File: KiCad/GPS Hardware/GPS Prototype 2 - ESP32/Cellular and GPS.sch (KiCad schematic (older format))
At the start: 30 parts, among them J3 Conn_Coaxial, J6 SIM8065-6-1-14-01-A_REVA1, Q1 BC847, Q2 BC847, Q3 BSS84, U10 ublox_SAM-M8Q, U7 74AVC2T245GU-Q100X, U8 SARA-U201

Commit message: Update
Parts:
- D2: symbol GPS-Hardware-rescue:LED-Device -> GPS-Hardware-rescue:LED-Device-GPS-Hardware-rescue
- D3, D4, D5, D6: symbol GPS-Hardware-rescue:D_TVS-Device -> GPS-Hardware-rescue:D_TVS-Device-GPS-Hardware-rescue
- J3: symbol GPS-Hardware-rescue:Conn_Coaxial-Connector -> GPS-Hardware-rescue:Conn_Coaxial-Connector-GPS-Hardware-rescue
- Q1, Q2: symbol GPS-Hardware-rescue:BC847-Transistor_BJT -> GPS-Hardware-rescue:BC847-Transistor_BJT-GPS-Hardware-rescue
- Q3: symbol GPS-Hardware-rescue:BSS84-Transistor_FET -> GPS-Hardware-rescue:BSS84-Transistor_FET-GPS-Hardware-rescue
- U10: symbol GPS-Hardware-rescue:ublox_SAM-M8Q-RF_GPS -> GPS-Hardware-rescue:ublox_SAM-M8Q-RF_GPS-GPS-Hardware-rescue
- U8: symbol GPS-Hardware-rescue:SARA-U201-RF_GSM -> GPS-Hardware-rescue:SARA-U201-RF_GSM-GPS-Hardware-rescue
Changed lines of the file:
@@
 $EndDescr
 $Comp
-L GPS-Hardware-rescue:SARA-U201-RF_GSM U?
+L GPS-Hardware-rescue:SARA-U201-RF_GSM-GPS-Hardware-rescue U?
 U 1 1 6149258C
 P 3100 2850
@@
 CTS_Cellular
 $Comp
-L GPS-Hardware-rescue:GND-power #PWR?
+L GPS-Hardware-rescue:GND-power-GPS-Hardware-rescue #PWR?
 U 1 1 61492596
 P 2500 1950
@@
 $EndComp
 $Comp
-L GPS-Hardware-rescue:+1V8-power #PWR?
+L GPS-Hardware-rescue:+1V8-power-GPS-Hardware-rescue #PWR?
 U 1 1 6149259C
 P 3200 1750
@@
 	1600 2850 1700 2850
 $Comp
-L GPS-Hardware-rescue:+3V3-power #PWR?
+L GPS-Hardware-rescue:+3V3-power-GPS-Hardware-rescue #PWR?
 U 1 1 614925A6
 P 1700 2550
@@
 VCC
 $Comp
-L GPS-Hardware-rescue:GND-power #PWR?
+L GPS-Hardware-rescue:GND-power-GPS-Hardware-rescue #PWR?
 U 1 1 614925D1
 P 1850 1500
@@
 $EndComp
 $Comp
-L GPS-Hardware-rescue:GND-power #PWR?
+L GPS-Hardware-rescue:GND-power-GPS-Hardware-rescue #PWR?
 U 1 1 614925D7
 P 2150 1500
@@
 $EndComp
 $Comp
-L GPS-Hardware-rescue:GND-power #PWR?
+L GPS-Hardware-rescue:GND-power-GPS-Hardware-rescue #PWR?
 U 1 1 614925DD
 P 2450 1500
@@
 $EndComp
 $Comp
-L GPS-Hardware-rescue:GND-power #PWR?
+L GPS-Hardware-rescue:GND-power-GPS-Hardware-rescue #PWR?
 U 1 1 614925E3
 P 2750 1500
@@
 VCC
 $Comp
-L GPS-Hardware-rescue:Conn_Coaxial-Connector J?
+L GPS-Hardware-rescue:Conn_Coaxial-Connector-GPS-Hardware-rescue J?
 U 1 1 614925ED
 P 3900 1950
@@
 $EndComp
 $Comp
-L GPS-Hardware-rescue:ublox_SAM-M8Q-RF_GPS U10
+L GPS-Hardware-rescue:ublox_SAM-M8Q-RF_GPS-GPS-Hardware-rescue U10
 U 1 1 614F3B93
 P 6000 6250
@@
 $EndComp
 $Comp
-L GPS-Hardware-rescue:GND-power #PWR0171
+L GPS-Hardware-rescue:GND-power-GPS-Hardware-rescue #PWR0171
 U 1 1 6152BD4B
 P 2300 5800
@@
 $EndComp
 $Comp
-L GPS-Hardware-rescue:GND-power #PWR0172
+L GPS-Hardware-rescue:GND-power-GPS-Hardware-rescue #PWR0172
 U 1 1 6152F81D
 P 2300 5600
@@
 $EndComp
 $Comp
-L GPS-Hardware-rescue:GND-power #PWR0173
+L GPS-Hardware-rescue:GND-power-GPS-Hardware-rescue #PWR0173
 U 1 1 6153C648
 P 3300 6000
@@
 	3200 5700 3300 5700
 $Comp
-L GPS-Hardware-rescue:+1V8-power #PWR0174
+L GPS-Hardware-rescue:+1V8-power-GPS-Hardware-rescue #PWR0174
 U 1 1 6153DDB4
 P 3400 5700
@@
 	3200 5600 3950 5600
 $Comp
-L GPS-Hardware-rescue:GND-power #PWR0175
+L GPS-Hardware-rescue:GND-power-GPS-Hardware-rescue #PWR0175
 U 1 1 61540A2C
 P 3950 5900
@@
 Connection ~ 3950 5600
 $Comp
-L GPS-Hardware-rescue:GND-power #PWR0176
+L GPS-Hardware-rescue:GND-power-GPS-Hardware-rescue #PWR0176
 U 1 1 61553C2B
 P 3200 6250
@@
 TX_GPS
 $Comp
-L GPS-Hardware-rescue:GND-power #PWR0177
+L GPS-Hardware-rescue:GND-power-GPS-Hardware-rescue #PWR0177
 U 1 1 61577124
 P 6000 6750
@@
 $EndComp
 $Comp
-L GPS-Hardware-rescue:GND-power #PWR0178
+L GPS-Hardware-rescue:GND-power-GPS-Hardware-rescue #PWR0178
 U 1 1 61579240
 P 5600 5700
@@
 NoConn ~ 2500 3750
 $Comp
-L GPS-Hardware-rescue:GND-power #PWR0179
+L GPS-Hardware-rescue:GND-power-GPS-Hardware-rescue #PWR0179
 U 1 1 615C3FBF
 P 3100 3950
@@
 $EndComp
 $Comp
-L GPS-Hardware-rescue:BC847-Transistor_BJT Q1
+L GPS-Hardware-rescue:BC847-Transistor_BJT-GPS-Hardware-rescue Q1
 U 1 1 615DCAB0
 P 4350 2850
@@
 $EndComp
 $Comp
-L GPS-Hardware-rescue:LED-Device D2
+L GPS-Hardware-rescue:LED-Device-GPS-Hardware-rescue D2
 U 1 1 615DFC25
 P 4450 2500
@@
 	3750 2850 3700 2850
 $Comp
-L GPS-Hardware-rescue:GND-power #PWR0180
+L GPS-Hardware-rescue:GND-power-GPS-Hardware-rescue #PWR0180
 U 1 1 615E6884
 P 4450 3050
@@
 $EndComp
 $Comp
-L GPS-Hardware-rescue:GND-power #PWR0181
+L GPS-Hardware-rescue:GND-power-GPS-Hardware-rescue #PWR0181
 U 1 1 615E6F5B
 P 4100 3150
@@
 VSIM
 $Comp
-L GPS-Hardware-rescue:GND-power #PWR0113
+L GPS-Hardware-rescue:GND-power-GPS-Hardware-rescue #PWR0113
 U 1 1 61244203
 P 3900 1750
@@
 $EndComp
 $Comp
-L GPS-Hardware-rescue:GND-power #PWR0114
+L GPS-Hardware-rescue:GND-power-GPS-Hardware-rescue #PWR0114
 U 1 1 61320761
 P 7850 4250
@@
 $EndComp
 $Comp
-L GPS-Hardware-rescue:GND-power #PWR0128
+L GPS-Hardware-rescue:GND-power-GPS-Hardware-rescue #PWR0128
 U 1 1 61320767
 P 8350 4450
@@
 $EndComp
 $Comp
-L GPS-Hardware-rescue:GND-power #PWR0129
+L GPS-Hardware-rescue:GND-power-GPS-Hardware-rescue #PWR0129
 U 1 1 6132076D
 P 8250 5300
@@
 $EndComp
 $Comp
-L GPS-Hardware-rescue:GND-power #PWR0133
+L GPS-Hardware-rescue:GND-power-GPS-Hardware-rescue #PWR0133
 U 1 1 61320773
 P 7550 4350
@@
 $EndComp
 $Comp
-L GPS-Hardware-rescue:GND-power #PWR0157
+L GPS-Hardware-rescue:GND-power-GPS-Hardware-rescue #PWR0157
 U 1 1 61320779
 P 8200 4250
@@
 $EndComp
 $Comp
-L GPS-Hardware-rescue:GND-power #PWR0158
+L GPS-Hardware-rescue:GND-power-GPS-Hardware-rescue #PWR0158
 U 1 1 6132077F
 P 7950 5500
@@
 RST
 $Comp
-L GPS-Hardware-rescue:D_TVS-Device D3
+L GPS-Hardware-rescue:D_TVS-Device-GPS-Hardware-rescue D3
 U 1 1 61320797
 P 7850 4100
@@
 $EndComp
 $Comp
-L GPS-Hardware-rescue:D_TVS-Device D5
+L GPS-Hardware-rescue:D_TVS-Device-GPS-Hardware-rescue D5
 U 1 1 6132079D
 P 8250 5150
@@
 $EndComp
 $Comp
-L GPS-Hardware-rescue:D_TVS-Device D4
+L GPS-Hardware-rescue:D_TVS-Device-GPS-Hardware-rescue D4
 U 1 1 613207AF
 P 8350 4600
@@
 VSIM
 $Comp
-L GPS-Hardware-rescue:GND-power #PWR0159
+L GPS-Hardware-rescue:GND-power-GPS-Hardware-rescue #PWR0159
 U 1 1 61330E52
 P 8000 3550
@@
 $EndComp
 $Comp
-L GPS-Hardware-rescue:GND-power #PWR0160
+L GPS-Hardware-rescue:GND-power-GPS-Hardware-rescue #PWR0160
 U 1 1 61330E58
 P 7700 3550
@@
 $EndComp
 $Comp
-L GPS-Hardware-rescue:GND-power #PWR0161
+L GPS-Hardware-rescue:GND-power-GPS-Hardware-rescue #PWR0161
 U 1 1 61330E5E
 P 7350 3550
@@
 Connection ~ 8000 3850
 $Comp
-L GPS-Hardware-rescue:D_TVS-Device D6
+L GPS-Hardware-rescue:D_TVS-Device-GPS-Hardware-rescue D6
 U 1 1 61330E66
 P 8000 3700
@@
 $EndComp
 $Comp
-L GPS-Hardware-rescue:GND-power #PWR0162
+L GPS-Hardware-rescue:GND-power-GPS-Hardware-rescue #PWR0162
 U 1 1 61331880
 P 8650 4150
@@
 $EndComp
 $Comp
-L GPS-Hardware-rescue:BC847-Transistor_BJT Q2
+L GPS-Hardware-rescue:BC847-Transistor_BJT-GPS-Hardware-rescue Q2
 U 1 1 613C6B7F
 P 5050 4050
@@
 	4750 4050 4850 4050
 $Comp
-L GPS-Hardware-rescue:GND-power #PWR0104
+L GPS-Hardware-rescue:GND-power-GPS-Hardware-rescue #PWR0104
 U 1 1 613D3752
 P 5150 4350
@@
 	5150 3750 5150 3800
 $Comp
-L GPS-Hardware-rescue:+3V3-power #PWR0163
+L GPS-Hardware-rescue:+3V3-power-GPS-Hardware-rescue #PWR0163
 U 1 1 613DE378
 P 5150 3350
@@
 	5150 3450 5150 3350
 $Comp
-L GPS-Hardware-rescue:BSS84-Transistor_FET Q3
+L GPS-Hardware-rescue:BSS84-Transistor_FET-GPS-Hardware-rescue Q3
 U 1 1 613E1FB9
 P 5650 3800

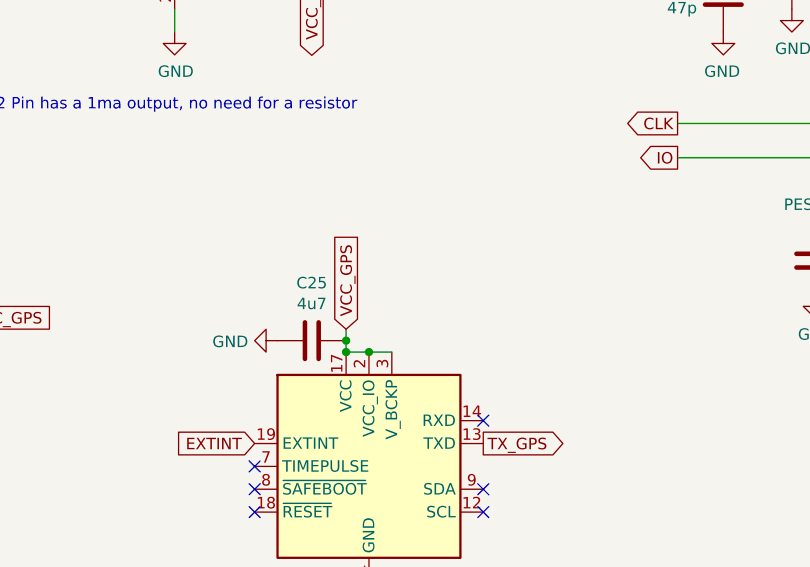
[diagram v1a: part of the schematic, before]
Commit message: Update to Laptop
Still a lot more to go
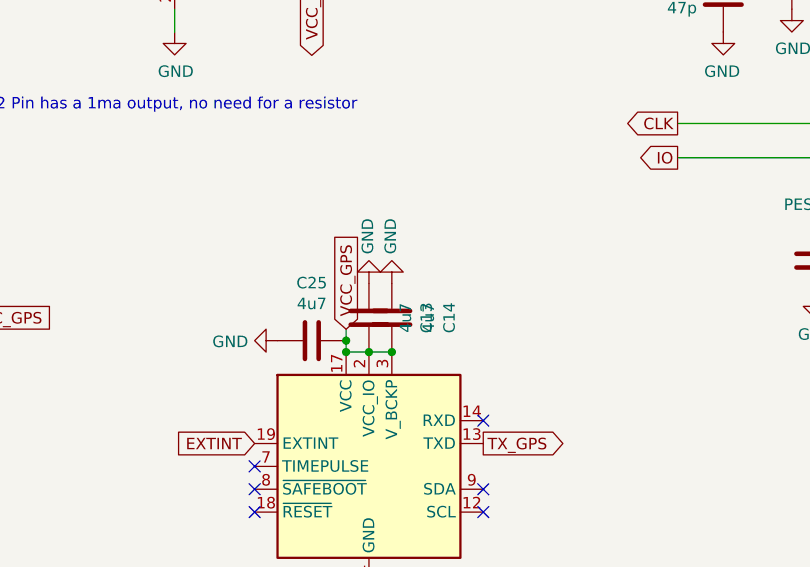
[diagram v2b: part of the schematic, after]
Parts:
- added C13, C14: 4u7, Capacitor_SMD:C_1206_3216Metric_Pad1.33x1.80mm_HandSolder, symbol GPS-Hardware-rescue:C-Device
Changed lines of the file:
@@
 NoConn ~ 8650 4450
 NoConn ~ 8650 4250
+$Comp
+L GPS-Hardware-rescue:C-Device C13
+U 1 1 62C636CA
+P 6000 5600
+F 0 "C13" V 5748 5600 50  0000 C CNN
+F 1 "4u7" V 5839 5600 50  0000 C CNN
+F 2 "Capacitor_SMD:C_1206_3216Metric_Pad1.33x1.80mm_HandSolder" H 6038 5450 50  0001 C CNN
+F 3 "~" H 6000 5600 50  0001 C CNN
+	1    6000 5600
+	-1   0    0    1
+$EndComp
+$Comp
+L GPS-Hardware-rescue:C-Device C14
+U 1 1 62C6483D
+P 6100 5600
+F 0 "C14" V 5848 5600 50  0000 C CNN
+F 1 "4u7" V 5939 5600 50  0000 C CNN
+F 2 "Capacitor_SMD:C_1206_3216Metric_Pad1.33x1.80mm_HandSolder" H 6138 5450 50  0001 C CNN
+F 3 "~" H 6100 5600 50  0001 C CNN
+	1    6100 5600
+	-1   0    0    1
+$EndComp
+Connection ~ 6100 5750
+$Comp
+L GPS-Hardware-rescue:GND-power-GPS-Hardware-rescue #PWR07
+U 1 1 62C65505
+P 6000 5450
+F 0 "#PWR07" H 6000 5200 50  0001 C CNN
+F 1 "GND" V 6005 5322 50  0000 R CNN
+F 2 "" H 6000 5450 50  0001 C CNN
+F 3 "" H 6000 5450 50  0001 C CNN
+	1    6000 5450
+	-1   0    0    1
+$EndComp
+$Comp
+L GPS-Hardware-rescue:GND-power-GPS-Hardware-rescue #PWR08
+U 1 1 62C65DF6
+P 6100 5450
+F 0 "#PWR08" H 6100 5200 50  0001 C CNN
+F 1 "GND" V 6105 5322 50  0000 R CNN
+F 2 "" H 6100 5450 50  0001 C CNN
+F 3 "" H 6100 5450 50  0001 C CNN
+	1    6100 5450
+	-1   0    0    1
+$EndComp
 $EndSCHEMATC

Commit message: Update to laptop
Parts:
- removed D3, D4, D5, D6: PESD0402, Capacitor_SMD:C_0402_1005Metric_Pad0.74x0.62mm_HandSolder, symbol GPS-Hardware-rescue:D_TVS-Device-GPS-Hardware-rescue
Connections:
- wire segments 50 -> 45
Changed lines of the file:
@@
-$EndComp
-$Comp
-L GPS-Hardware-rescue:GND-power-GPS-Hardware-rescue #PWR0114
-U 1 1 61320761
-P 7850 4250
-F 0 "#PWR0114" H 7850 4000 50  0001 C CNN
-F 1 "GND" H 7855 4077 50  0000 C CNN
-F 2 "" H 7850 4250 50  0001 C CNN
-F 3 "" H 7850 4250 50  0001 C CNN
-	1    7850 4250
-	1    0    0    -1
-$EndComp
-$Comp
-L GPS-Hardware-rescue:GND-power-GPS-Hardware-rescue #PWR0128
-U 1 1 61320767
-P 8350 4450
-F 0 "#PWR0128" H 8350 4200 50  0001 C CNN
-F 1 "GND" H 8355 4277 50  0000 C CNN
-F 2 "" H 8350 4450 50  0001 C CNN
-F 3 "" H 8350 4450 50  0001 C CNN
-	1    8350 4450
-	-1   0    0    1
-$EndComp
-$Comp
-L GPS-Hardware-rescue:GND-power-GPS-Hardware-rescue #PWR0129
-U 1 1 6132076D
-P 8250 5300
-F 0 "#PWR0129" H 8250 5050 50  0001 C CNN
-F 1 "GND" H 8255 5127 50  0000 C CNN
-F 2 "" H 8250 5300 50  0001 C CNN
-F 3 "" H 8250 5300 50  0001 C CNN
-	1    8250 5300
-	1    0    0    -1
 $EndComp
 $Comp
@@
 Connection ~ 7550 3950
 Wire Wire Line
-	8250 5000 8250 4900
-Wire Wire Line
-	8250 4900 7950 4900
-Connection ~ 8250 4900
-Wire Wire Line
 	7950 5200 7950 4900
 Text GLabel 7350 4750 0    50   Output ~ 0
@@
 Text GLabel 7350 3950 0    50   Output ~ 0
 RST
-$Comp
-L GPS-Hardware-rescue:D_TVS-Device-GPS-Hardware-rescue D3
-U 1 1 61320797
-P 7850 4100
-F 0 "D3" V 7804 4180 50  0000 L CNN
-F 1 "PESD0402" V 7895 4180 50  0000 L CNN
-F 2 "Capacitor_SMD:C_0402_1005Metric_Pad0.74x0.62mm_HandSolder" H 7850 4100 50  0001 C CNN
-F 3 "~" H 7850 4100 50  0001 C CNN
-	1    7850 4100
-	0    -1   -1   0
-$EndComp
-$Comp
-L GPS-Hardware-rescue:D_TVS-Device-GPS-Hardware-rescue D5
-U 1 1 6132079D
-P 8250 5150
-F 0 "D5" V 8204 5230 50  0000 L CNN
-F 1 "PESD0402" V 8295 5230 50  0000 L CNN
-F 2 "Capacitor_SMD:C_0402_1005Metric_Pad0.74x0.62mm_HandSolder" H 8250 5150 50  0001 C CNN
-F 3 "~" H 8250 5150 50  0001 C CNN
-	1    8250 5150
-	0    -1   -1   0
-$EndComp
 $Comp
 L GPS-Hardware-rescue:C-Device C28
@@
 	1    7950 5350
 	1    0    0    -1
-$EndComp
-$Comp
-L GPS-Hardware-rescue:D_TVS-Device-GPS-Hardware-rescue D4
-U 1 1 613207AF
-P 8350 4600
-F 0 "D4" V 8304 4680 50  0000 L CNN
-F 1 "PESD0402" V 8395 4680 50  0000 L CNN
-F 2 "Capacitor_SMD:C_0402_1005Metric_Pad0.74x0.62mm_HandSolder" H 8350 4600 50  0001 C CNN
-F 3 "~" H 8350 4600 50  0001 C CNN
-	1    8350 4600
-	0    1    1    0
 $EndComp
 $Comp
@@
 VSIM
 $Comp
-L GPS-Hardware-rescue:GND-power-GPS-Hardware-rescue #PWR0159
-U 1 1 61330E52
-P 8000 3550
-F 0 "#PWR0159" H 8000 3300 50  0001 C CNN
-F 1 "GND" H 8005 3377 50  0000 C CNN
-F 2 "" H 8000 3550 50  0001 C CNN
-F 3 "" H 8000 3550 50  0001 C CNN
-	1    8000 3550
-	1    0    0    1
-$EndComp
-$Comp
 L GPS-Hardware-rescue:GND-power-GPS-Hardware-rescue #PWR0160
 U 1 1 61330E58
@@
 	1    0    0    1
 $EndComp
-Connection ~ 8000 3850
-$Comp
-L GPS-Hardware-rescue:D_TVS-Device-GPS-Hardware-rescue D6
-U 1 1 61330E66
-P 8000 3700
-F 0 "D6" V 7954 3780 50  0000 L CNN
-F 1 "PESD0402" V 8045 3780 50  0000 L CNN
-F 2 "Capacitor_SMD:C_0402_1005Metric_Pad0.74x0.62mm_HandSolder" H 8000 3700 50  0001 C CNN
-F 3 "~" H 8000 3700 50  0001 C CNN
-	1    8000 3700
-	0    1    -1   0
-$EndComp
 $Comp
 L GPS-Hardware-rescue:C-Device C31
@@
 	1    0    0    1
 $EndComp
-Wire Wire Line
-	7700 3850 8000 3850
 Wire Wire Line
 	7350 3850 7700 3850
@@
 $EndComp
 Wire Wire Line
-	8000 3850 8650 3850
-Connection ~ 7850 3950
-Wire Wire Line
-	7850 3950 7550 3950
-Wire Wire Line
-	7850 3950 8650 3950
-Wire Wire Line
 	7350 4750 8200 4750
 Wire Wire Line
@@
 Connection ~ 8200 4750
 Wire Wire Line
-	8200 4750 8350 4750
-Wire Wire Line
-	8350 4750 8500 4750
-Wire Wire Line
 	8500 4750 8500 4050
 Wire Wire Line
 	8500 4050 8650 4050
-Connection ~ 8350 4750
 Connection ~ 7950 4900
 Wire Wire Line
@@
 Wire Wire Line
 	8600 4350 8650 4350
-Wire Wire Line
-	8250 4900 8600 4900
 NoConn ~ 8650 4450
 NoConn ~ 8650 4250
@@
 	-1   0    0    1
 $EndComp
+Wire Wire Line
+	7700 3850 8650 3850
+Wire Wire Line
+	7550 3950 8650 3950
+Wire Wire Line
+	8200 4750 8500 4750
+Wire Wire Line
+	7950 4900 8600 4900
 $EndSCHEMATC

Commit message: Update
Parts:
- removed Q2: BC847, Package_TO_SOT_SMD:SOT-23, symbol GPS-Hardware-rescue:BC847-Transistor_BJT-GPS-Hardware-rescue
- removed Q3: BSS84, Package_TO_SOT_SMD:SOT-323_SC-70, symbol GPS-Hardware-rescue:BSS84-Transistor_FET-GPS-Hardware-rescue
- removed R20: 47k, Resistor_SMD:R_1206_3216Metric_Pad1.30x1.75mm_HandSolder, symbol GPS-Hardware-rescue:R-Device
- added D3: LED, LED_SMD:LED_1206_3216Metric_Pad1.42x1.75mm_HandSolder, symbol Device:LED
- added Q2: 2N7002, Package_TO_SOT_SMD:SOT-23, symbol Transistor_FET:2N7002
- added R15: 1k, Resistor_SMD:R_1206_3216Metric_Pad1.30x1.75mm_HandSolder, symbol Device:R
- R19: value 250 -> 820
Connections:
- net labels removed: GPIO2, VCC_GPS
- wire segments 45 -> 39
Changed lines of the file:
@@
 	1    0    0    -1
 $EndComp
-Text GLabel 2500 3050 0    50   Output ~ 0
+Text GLabel 1400 3250 0    50   Output ~ 0
 RESET_Cellular
 Wire Wire Line
@@
 	1    0    0    -1
 $EndComp
-Text GLabel 3700 2950 2    50   Output ~ 0
-GPIO2
 $Comp
 L GPS~Hardware:74AVC2T245GU-Q100X U7
@@
 	0    1    1    0
 $EndComp
-Text GLabel 1900 5500 1    50   Input ~ 0
-VCC_GPS
 Wire Wire Line
 	1900 5500 1900 5700
@@
 	1    0    0    -1
 $EndComp
-Text GLabel 4200 5600 2    50   Input ~ 0
-VCC_GPS
 Wire Wire Line
 	4200 5600 3950 5600
@@
 Wire Wire Line
 	5900 5700 5900 5750
-Text GLabel 5900 5650 1    50   Input ~ 0
-VCC_GPS
 Wire Wire Line
 	6100 5750 6000 5750
@@
 Connection ~ 6000 5750
 Connection ~ 5900 5750
-NoConn ~ 5500 6250
 NoConn ~ 5500 6350
 NoConn ~ 5500 6450
@@
 AR Path="/613BCFF5/615E2B7B" Ref="R19"  Part="1"
 F 0 "R19" H 4520 2246 50  0000 L CNN
-F 1 "250" V 4450 2150 50  0000 L CNN
+F 1 "820" V 4450 2150 50  0000 L CNN
 F 2 "Resistor_SMD:R_1206_3216Metric_Pad1.30x1.75mm_HandSolder" V 4380 2200 50  0001 C CNN
 F 3 "~" H 4450 2200 50  0001 C CNN
@@
 	0    1    1    0
 $EndComp
-$Comp
-L GPS-Hardware-rescue:BC847-Transistor_BJT-GPS-Hardware-rescue Q2
-U 1 1 613C6B7F
-P 5050 4050
-F 0 "Q2" H 5241 4096 50  0000 L CNN
-F 1 "BC847" H 5241 4005 50  0000 L CNN
-F 2 "Package_TO_SOT_SMD:SOT-23" H 5250 3975 50  0001 L CIN
-F 3 "https://www.mouser.co.uk/datasheet/2/308/1/BC846ALT1_D-2310268.pdf" H 5050 4050 50  0001 L CNN
-	1    5050 4050
-	1    0    0    -1
-$EndComp
-Text GLabel 4750 4050 0    50   Input ~ 0
-GPIO2
-Wire Wire Line
-	4750 4050 4850 4050
-$Comp
-L GPS-Hardware-rescue:GND-power-GPS-Hardware-rescue #PWR0104
-U 1 1 613D3752
-P 5150 4350
-F 0 "#PWR0104" H 5150 4100 50  0001 C CNN
-F 1 "GND" H 5155 4177 50  0000 C CNN
-F 2 "" H 5150 4350 50  0001 C CNN
-F 3 "" H 5150 4350 50  0001 C CNN
-	1    5150 4350
-	1    0    0    -1
-$EndComp
-Wire Wire Line
-	5150 4250 5150 4350
-$Comp
-L GPS-Hardware-rescue:R-Device R20
-U 1 1 613D777A
-P 5150 3600
-F 0 "R20" H 5220 3646 50  0000 L CNN
-F 1 "47k" H 5220 3555 50  0000 L CNN
-F 2 "Resistor_SMD:R_1206_3216Metric_Pad1.30x1.75mm_HandSolder" V 5080 3600 50  0001 C CNN
-F 3 "~" H 5150 3600 50  0001 C CNN
-	1    5150 3600
-	1    0    0    -1
-$EndComp
-Wire Wire Line
-	5150 3750 5150 3800
-$Comp
-L GPS-Hardware-rescue:+3V3-power-GPS-Hardware-rescue #PWR0163
-U 1 1 613DE378
-P 5150 3350
-F 0 "#PWR0163" H 5150 3200 50  0001 C CNN
-F 1 "+3V3" H 5165 3523 50  0000 C CNN
-F 2 "" H 5150 3350 50  0001 C CNN
-F 3 "" H 5150 3350 50  0001 C CNN
-	1    5150 3350
-	1    0    0    -1
-$EndComp
-Wire Wire Line
-	5150 3450 5150 3350
-$Comp
-L GPS-Hardware-rescue:BSS84-Transistor_FET-GPS-Hardware-rescue Q3
-U 1 1 613E1FB9
-P 5650 3800
-F 0 "Q3" H 5854 3754 50  0000 L CNN
-F 1 "BSS84" H 5854 3845 50  0000 L CNN
-F 2 "Package_TO_SOT_SMD:SOT-323_SC-70" H 5850 3725 50  0001 L CIN
-F 3 "http://assets.nexperia.com/documents/data-sheet/BSS84.pdf" H 5650 3800 50  0001 L CNN
-	1    5650 3800
-	1    0    0    1
-$EndComp
-Wire Wire Line
-	5450 3800 5150 3800
-Connection ~ 5150 3800
-Wire Wire Line
-	5150 3800 5150 3850
-Wire Wire Line
-	5150 3450 5750 3450
-Wire Wire Line
-	5750 3450 5750 3600
-Connection ~ 5150 3450
-Text GLabel 5750 4050 3    50   Output ~ 0
-VCC_GPS
-Wire Wire Line
-	5750 4000 5750 4050
-Text Notes 4200 4700 0    50   ~ 0
+Text Notes 5050 2850 0    50   ~ 0
 GPIO2 Pin has a 1ma output, no need for a resistor
 $Comp
@@
 Wire Wire Line
 	7950 4900 8600 4900
+NoConn ~ 3700 2950
+$Comp
+L GPS-Hardware-rescue:+3V3-power-GPS-Hardware-rescue #PWR?
+U 1 1 62EFB8D4
+P 1900 5500
+AR Path="/613BCFBA/62EFB8D4" Ref="#PWR?"  Part="1"
+AR Path="/613BCFF5/62EFB8D4" Ref="#PWR0114"  Part="1"
+F 0 "#PWR0114" H 1900 5350 50  0001 C CNN
+F 1 "+3V3" H 1915 5673 50  0000 C CNN
+F 2 "" H 1900 5500 50  0001 C CNN
+F 3 "" H 1900 5500 50  0001 C CNN
+	1    1900 5500
+	1    0    0    -1
+$EndComp
+$Comp
+L GPS-Hardware-rescue:+3V3-power-GPS-Hardware-rescue #PWR?
+U 1 1 62EFC3B1
+P 5900 5650
+AR Path="/613BCFBA/62EFC3B1" Ref="#PWR?"  Part="1"
+AR Path="/613BCFF5/62EFC3B1" Ref="#PWR0124"  Part="1"
+F 0 "#PWR0124" H 5900 5500 50  0001 C CNN
+F 1 "+3V3" H 5915 5823 50  0000 C CNN
+F 2 "" H 5900 5650 50  0001 C CNN
+F 3 "" H 5900 5650 50  0001 C CNN
+	1    5900 5650
+	1    0    0    -1
+$EndComp
+$Comp
+L GPS-Hardware-rescue:+3V3-power-GPS-Hardware-rescue #PWR?
+U 1 1 62EFD51B
+P 4200 5600
+AR Path="/613BCFBA/62EFD51B" Ref="#PWR?"  Part="1"
+AR Path="/613BCFF5/62EFD51B" Ref="#PWR0125"  Part="1"
+F 0 "#PWR0125" H 4200 5450 50  0001 C CNN
+F 1 "+3V3" H 4215 5773 50  0000 C CNN
+F 2 "" H 4200 5600 50  0001 C CNN
+F 3 "" H 4200 5600 50  0001 C CNN
+	1    4200 5600
+	0    1    1    0
+$EndComp
+$Comp
+L Device:R R15
+U 1 1 62F08847
+P 5000 6250
+F 0 "R15" V 4793 6250 50  0000 C CNN
+F 1 "1k" V 4884 6250 50  0000 C CNN
+F 2 "Resistor_SMD:R_1206_3216Metric_Pad1.30x1.75mm_HandSolder" V 4930 6250 50  0001 C CNN
+F 3 "~" H 5000 6250 50  0001 C CNN
+	1    5000 6250
+	0    1    1    0
+$EndComp
+$Comp
+L Device:LED D3
+U 1 1 62F09DE8
+P 4650 6250
+F 0 "D3" H 4643 6467 50  0000 C CNN
+F 1 "LED" H 4643 6376 50  0000 C CNN
+F 2 "LED_SMD:LED_1206_3216Metric_Pad1.42x1.75mm_HandSolder" H 4650 6250 50  0001 C CNN
+F 3 "~" H 4650 6250 50  0001 C CNN
+	1    4650 6250
+	1    0    0    -1
+$EndComp
+$Comp
+L GPS-Hardware-rescue:GND-power-GPS-Hardware-rescue #PWR0126
+U 1 1 62F0AFD7
+P 4500 6250
+F 0 "#PWR0126" H 4500 6000 50  0001 C CNN
+F 1 "GND" V 4505 6122 50  0000 R CNN
+F 2 "" H 4500 6250 50  0001 C CNN
+F 3 "" H 4500 6250 50  0001 C CNN
+	1    4500 6250
+	0    1    1    0
+$EndComp
+Wire Wire Line
+	4800 6250 4850 6250
+Wire Wire Line
+	5150 6250 5500 6250
+$Comp
+L Transistor_FET:2N7002 Q2
+U 1 1 62F10032
+P 1600 3250
+F 0 "Q2" H 1804 3296 50  0000 L CNN
+F 1 "2N7002" H 1804 3205 50  0000 L CNN
+F 2 "Package_TO_SOT_SMD:SOT-23" H 1800 3175 50  0001 L CIN
+F 3 "https://www.onsemi.com/pub/Collateral/NDS7002A-D.PDF" H 1600 3250 50  0001 L CNN
+	1    1600 3250
+	1    0    0    -1
+$EndComp
+Wire Wire Line
+	1700 3050 2500 3050
+$Comp
+L GPS-Hardware-rescue:GND-power-GPS-Hardware-rescue #PWR?
+U 1 1 62F1930C
+P 1700 3450
+AR Path="/613BCFBA/62F1930C" Ref="#PWR?"  Part="1"
+AR Path="/613BCFF5/62F1930C" Ref="#PWR0128"  Part="1"
+F 0 "#PWR0128" H 1700 3200 50  0001 C CNN
+F 1 "GND" H 1705 3277 50  0000 C CNN
+F 2 "" H 1700 3450 50  0001 C CNN
+F 3 "" H 1700 3450 50  0001 C CNN
+	1    1700 3450
+	1    0    0    -1
+$EndComp
 $EndSCHEMATC
